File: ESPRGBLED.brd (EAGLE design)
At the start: 160 x 100 mm, 20 parts

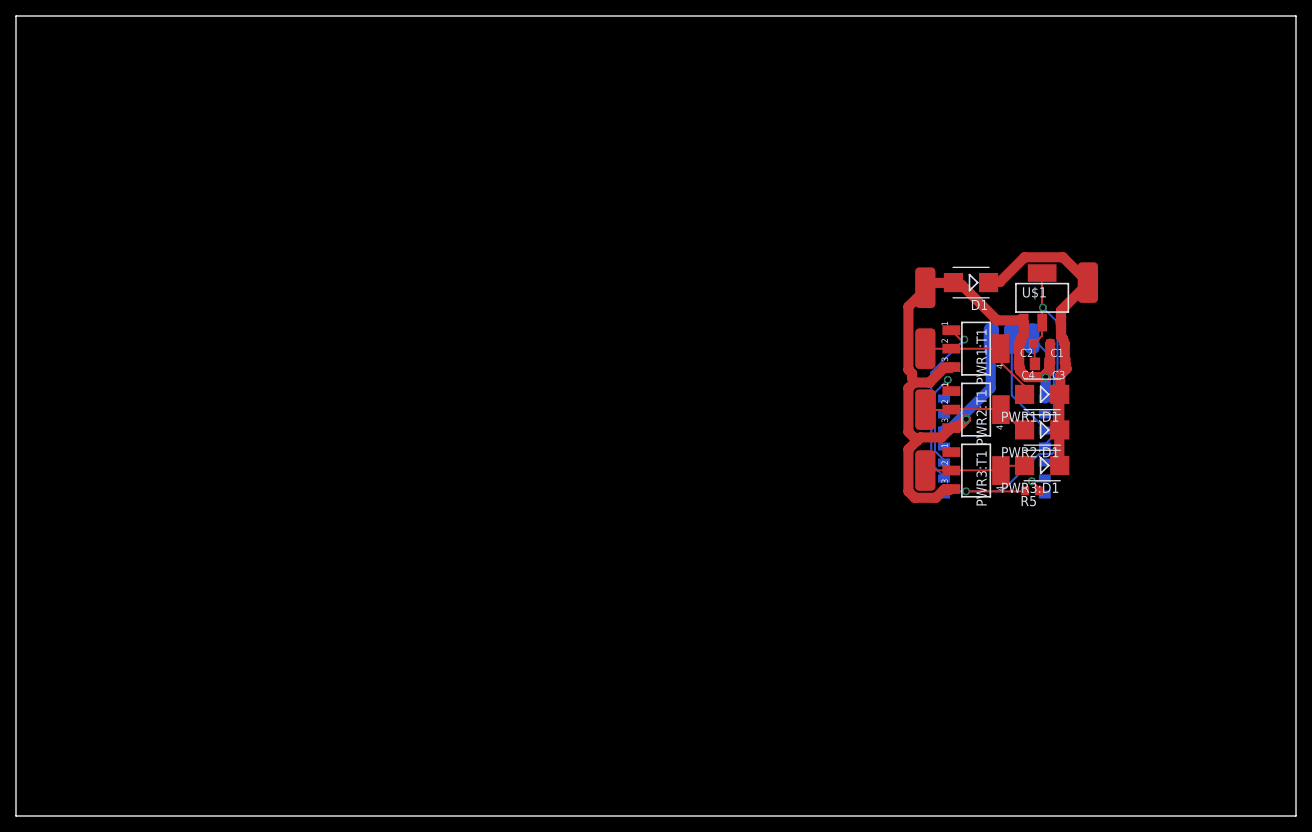
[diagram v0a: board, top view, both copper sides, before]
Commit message: layouted
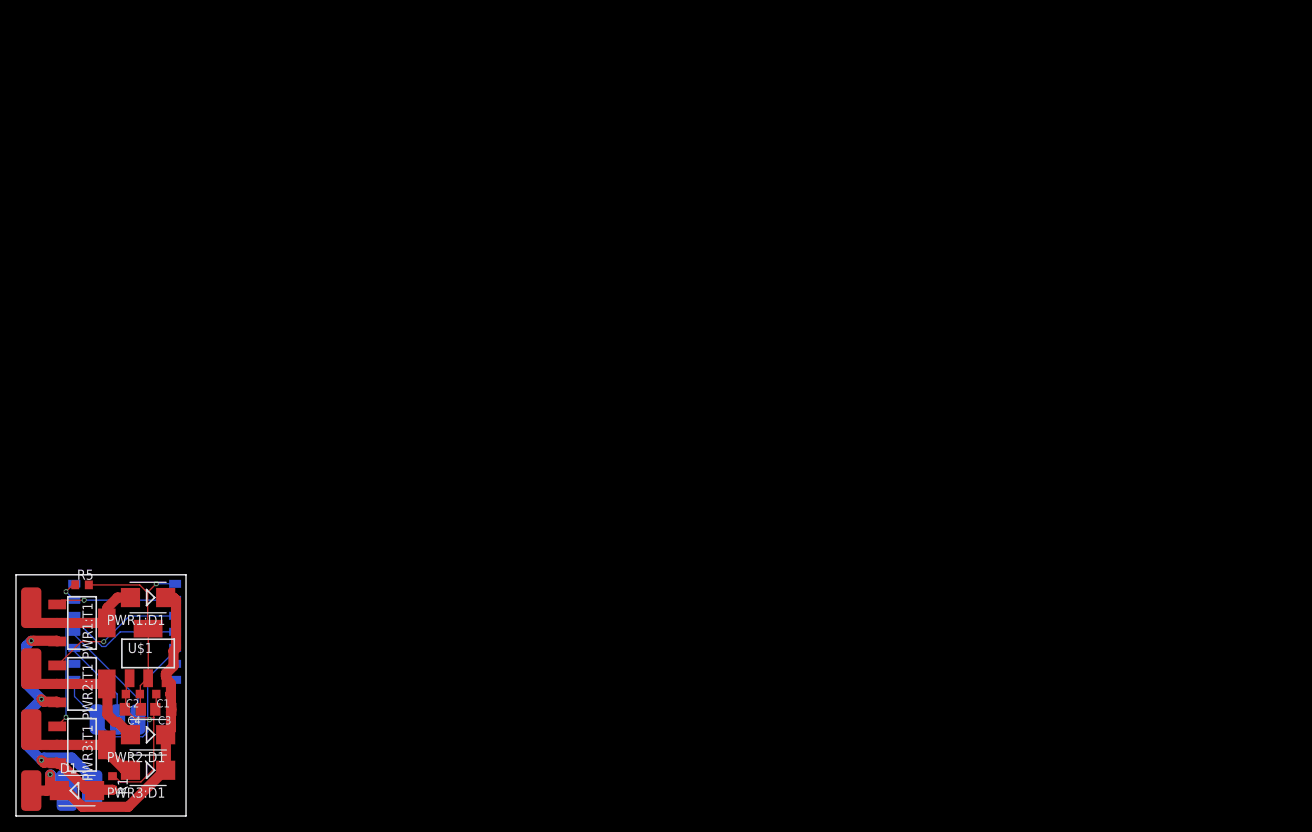
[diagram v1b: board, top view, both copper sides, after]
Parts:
- added R1: 0R, rcl:R0603
- added U$9: CON1, Fabian:CON1HP
- moved U$7 142.6 mm to (6.35, 3.17), flipped to the bottom, turned to 270 degrees
- moved D1 128.5 mm to (7.62, 3.17), turned to 0 degrees
- moved U$8 121.6 mm to (9.53, 3.17), flipped to the bottom
- moved U$3 121.5 mm to (12.7, 12.1)
- moved U$1 120.3 mm to (16.5, 20.3)
- moved C1 120.0 mm to (18.4, 15.2)
- moved C2 120.0 mm to (14.6, 15.2)
- moved C3 119.8 mm to (18.4, 13.3)
- moved C4 119.8 mm to (14.6, 13.3)
- moved R5 119.3 mm to (8.26, 28.9), turned to 0 degrees
- moved PWR2:D1 118.1 mm to (16.5, 10.2)
- moved PWR3:D1 118.1 mm to (16.5, 5.71)
- moved PWR1:T1 116.9 mm to (8.26, 24.1)
- moved PWR3:T1 116.9 mm to (8.26, 8.89)
- moved PWR2:T1 116.9 mm to (8.26, 16.5)
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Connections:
- new net DGND: C1.2, C2.2, C3.2, C4.2, R1.1, U$1.LEFT, U$2.GND, U$2.GPIO15, U$3.0V
- net +12V: now also U$9.P$1
- net GND: now also R1.2; no longer C1.2, C2.2, C3.2, C4.2, U$1.LEFT, U$2.GND, U$2.GPIO15, U$3.0V
- net N$2: now also U$2.GPIO13
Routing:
- net GND: track 92.8 -> 42.5 mm, vias 2 -> 3
- net DGND: track 0.00 -> 50.1 mm, vias 0 -> 1
- net N$2: track 0.00 -> 28.5 mm, vias 0 -> 1
- net VCC: track 54.3 -> 26.9 mm, vias 2 -> 1
- net +12V: track 39.9 -> 49.0 mm, vias 0 -> 1
- net N$6: track 21.8 -> 15.0 mm
- net N$4: track 13.6 -> 18.8 mm
- net N$3: track 13.1 -> 17.3 mm
- net N$5: track 12.7 -> 15.6 mm
- net N$8: track 13.2 -> 11.2 mm
- net N$7: track 15.1 -> 14.3 mm
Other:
- board size 160 x 100 mm -> 21.3 x 30.1 mm
